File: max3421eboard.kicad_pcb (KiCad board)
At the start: 2 copper layers, 41.3 x 48.9 mm, 32 parts, among them J1 USB A, J2 USB MicroB, J3 1x10, J4 1x8, J5 1x8, J6 1x3, J7 Conn_01x04, U1 MAX3421E, U2 LP2985-3.3, U3 STMPS2141STR, Y1 12MHz

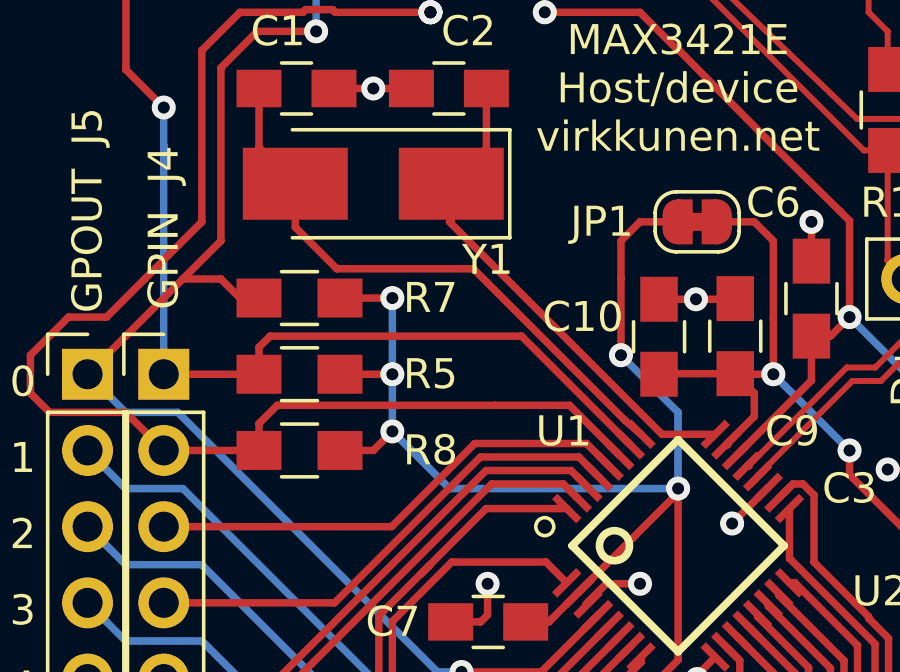
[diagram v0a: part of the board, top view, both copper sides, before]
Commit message: Clean-up
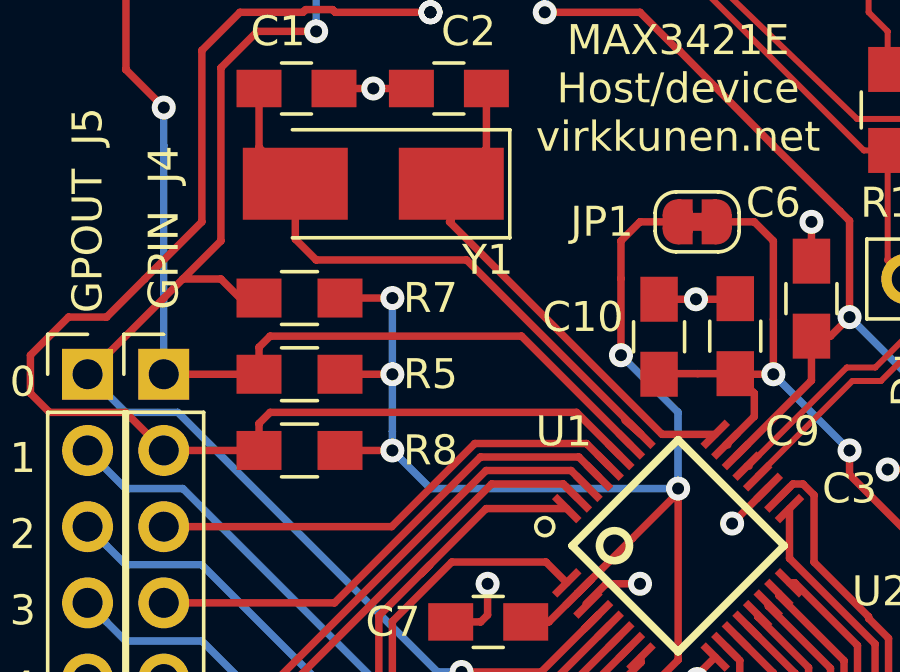
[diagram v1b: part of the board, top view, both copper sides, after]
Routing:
- net /X+: track 20.5 -> 21.4 mm
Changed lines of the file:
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@@
     (thickness 1.6)
     (drawings 47)
-    (tracks 460)
+    (tracks 458)
     (zones 0)
     (modules 32)
@@
   (segment (start 24.115 52.74) (end 22.235 54.62) (width 0.25) (layer F.Cu) (net 28))
   (segment (start 26.67 77.47) (end 23.495 77.47) (width 0.25) (layer F.Cu) (net 29))
-  (segment (start 38.695456 77.639796) (end 37.020659 75.964999) (width 0.25) (layer F.Cu) (net 29))
   (segment (start 26.67 76.57) (end 26.67 77.47) (width 0.25) (layer F.Cu) (net 29))
-  (segment (start 27.275001 75.964999) (end 26.67 76.57) (width 0.25) (layer F.Cu) (net 29))
-  (segment (start 34.525001 75.964999) (end 34.525001 75.964999) (width 0.25) (layer F.Cu) (net 29))
-  (segment (start 37.020659 75.964999) (end 34.525001 75.964999) (width 0.25) (layer F.Cu) (net 29))
-  (segment (start 34.525001 75.964999) (end 27.275001 75.964999) (width 0.25) (layer F.Cu) (net 29))
   (segment (start 32.385 62.865) (end 32.385 62.865) (width 0.25) (layer F.Cu) (net 29))
   (via (at 32.385 62.865) (size 0.8) (drill 0.4) (layers F.Cu B.Cu) (net 29))
@@
   (segment (start 28.136998 62.865) (end 28.226999 62.774999) (width 0.25) (layer F.Cu) (net 29))
   (segment (start 28.226999 62.774999) (end 29.119999 62.774999) (width 0.25) (layer F.Cu) (net 29))
+  (segment (start 26.67 76.57) (end 27.04 76.2) (width 0.25) (layer F.Cu) (net 29))
+  (segment (start 37.25566 76.2) (end 38.695456 77.639796) (width 0.25) (layer F.Cu) (net 29))
+  (segment (start 27.04 76.2) (end 37.25566 76.2) (width 0.25) (layer F.Cu) (net 29))
   (segment (start 32.217 53.285) (end 31.527 53.975) (width 0.25) (layer F.Cu) (net 30))
   (segment (start 32.217 52.71) (end 32.217 53.285) (width 0.25) (layer F.Cu) (net 30))
@@
   (segment (start 29.37 74.93) (end 29.845 74.93) (width 0.25) (layer F.Cu) (net 31))
   (segment (start 29.845 74.93) (end 31.115 74.93) (width 0.25) (layer F.Cu) (net 31))
-  (segment (start 29.37 77.47) (end 30.48 77.47) (width 0.25) (layer F.Cu) (net 31))
-  (segment (start 30.48 77.47) (end 31.115 76.835) (width 0.25) (layer F.Cu) (net 31))
-  (segment (start 31.115 76.835) (end 31.115 76.835) (width 0.25) (layer F.Cu) (net 31))
-  (via (at 31.115 76.835) (size 0.8) (drill 0.4) (layers F.Cu B.Cu) (net 31))
+  (via (at 31.115 77.47) (size 0.8) (drill 0.4) (layers F.Cu B.Cu) (net 31))
   (segment (start 31.115 74.93) (end 31.115 74.93) (width 0.25) (layer F.Cu) (net 31))
   (via (at 31.115 74.93) (size 0.8) (drill 0.4) (layers F.Cu B.Cu) (net 31))
@@
   (segment (start 40.64 76.2) (end 40.64 78.74) (width 0.25) (layer B.Cu) (net 31))
   (segment (start 38.735 74.295) (end 38.735 74.295) (width 0.25) (layer B.Cu) (net 31))
-  (segment (start 31.115 76.835) (end 33.02 78.74) (width 0.25) (layer B.Cu) (net 31))
   (segment (start 33.02 78.74) (end 40.64 78.74) (width 0.25) (layer B.Cu) (net 31))
   (segment (start 38.735 74.295) (end 40.64 76.2) (width 0.25) (layer B.Cu) (net 31))
@@
   (segment (start 39.37 69.85) (end 38.735 70.485) (width 0.25) (layer F.Cu) (net 31))
   (segment (start 40.625 69.85) (end 39.37 69.85) (width 0.25) (layer F.Cu) (net 31))
+  (segment (start 29.37 77.47) (end 31.115 77.47) (width 0.25) (layer F.Cu) (net 31))
+  (segment (start 31.115 76.835) (end 31.115 77.47) (width 0.25) (layer B.Cu) (net 31))
+  (segment (start 31.115 77.47) (end 32.385 78.74) (width 0.25) (layer B.Cu) (net 31))
+  (segment (start 32.385 78.74) (end 33.02 78.74) (width 0.25) (layer B.Cu) (net 31))
   (segment (start 47.625 67.47) (end 47.625 71.12) (width 0.2) (layer F.Cu) (net 32))
   (segment (start 42.938097 77.99335) (end 43.005963 77.99335) (width 0.25) (layer F.Cu) (net 32))
@@
   (segment (start 26.67 67.37) (end 27.88 68.58) (width 0.25) (layer F.Cu) (net 34))
   (segment (start 26.67 65.405) (end 26.67 67.37) (width 0.25) (layer F.Cu) (net 34))
-  (segment (start 33.817006 71.414999) (end 38.869326 76.467319) (width 0.25) (layer F.Cu) (net 34))
-  (segment (start 29.264999 71.414999) (end 33.817006 71.414999) (width 0.25) (layer F.Cu) (net 34))
-  (segment (start 27.88 68.58) (end 27.88 70.03) (width 0.25) (layer F.Cu) (net 34))
   (segment (start 38.869326 76.467319) (end 39.402563 76.932689) (width 0.25) (layer F.Cu) (net 34))
-  (segment (start 27.88 70.03) (end 29.264999 71.414999) (width 0.25) (layer F.Cu) (net 34))
+  (segment (start 27.88 68.58) (end 27.88 70.425) (width 0.25) (layer F.Cu) (net 34))
+  (segment (start 27.88 70.425) (end 28.575 71.12) (width 0.25) (layer F.Cu) (net 34))
+  (segment (start 33.589874 71.12) (end 39.402563 76.932689) (width 0.25) (layer F.Cu) (net 34))
+  (segment (start 28.575 71.12) (end 33.589874 71.12) (width 0.25) (layer F.Cu) (net 34))
   (segment (start 33.02 68.52) (end 33.08 68.58) (width 0.25) (layer F.Cu) (net 35))
   (segment (start 32.385 67.885) (end 33.08 68.58) (width 0.25) (layer F.Cu) (net 35))
